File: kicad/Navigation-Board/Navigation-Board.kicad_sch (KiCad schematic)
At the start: 178 parts, among them J1 2.8" TFT, J2 0.96" OLED, J3 GME0831B, J4 Conn_01x03, SW1 SW_SPST, SW10 SW_SPST, SW11 SW_SPST, SW12 SW_SPST, SW13 SW_SPST, SW14 SW_SPST, SW15 SW_SPST, SW16 SW_SPST, SW17 SW_SPST, SW18 SW_SPST, SW19 SW_SPST, SW2 SW_SPST, SW20 SW_SPST, SW21 SW_SPST, SW22 SW_SPST, SW23 SW_SPST, SW24 SW_SPST, SW25 SW_SPST, SW26 SW_SPST, SW27 SW_SPST, SW28 SW_SPST, SW29 SW_SPST, SW3 SW_SPST, SW30 SW_SPST, SW31 SW_SPST, SW32 SW_SPST, SW33 SW_SPST, SW34 SW_SPST, SW35 SW_SPST, SW36 SW_SPST, SW37 SW_SPST, SW38 SW_SPST, SW39 SW_SPST, SW4 SW_SPST, SW40 SW_SPST, SW41 SW_SPST, SW42 SW_SPST, SW43 SW_SPST, SW44 SW_SPST, SW45 SW_SPST, SW46 SW_SPST, SW47 SW_SPST, SW48 SW_SPST, SW49 SW_SPST, SW5 SW_SPST, SW50 SW_SPST, SW51 SW_SPST, SW52 SW_SPST, SW53 SW_SPST, SW54 SW_SPST, SW55 SW_SPST, SW56 SW_SPST, SW57 SW_SPST, SW58 SW_SPST, SW59 SW_SPST, SW6 SW_SPST, SW60 SW_SPST, SW61 SW_SPST, SW62 SW_SPST, SW63 SW_SPST, SW64 SW_SPST, SW65 SW_SPST, SW66 SW_SPST, SW67 SW_SPST, SW68 SW_SPST, SW69 SW_SPST, SW7 SW_SPST, SW70 SW_SPST, SW71 SW_SPST, SW72 SW_SPST, SW73 SW_SPST, SW74 SW_SPST, SW75 SW_SPST, SW76 SW_SPST, SW77 SW_SPST, SW78 SW_SPST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

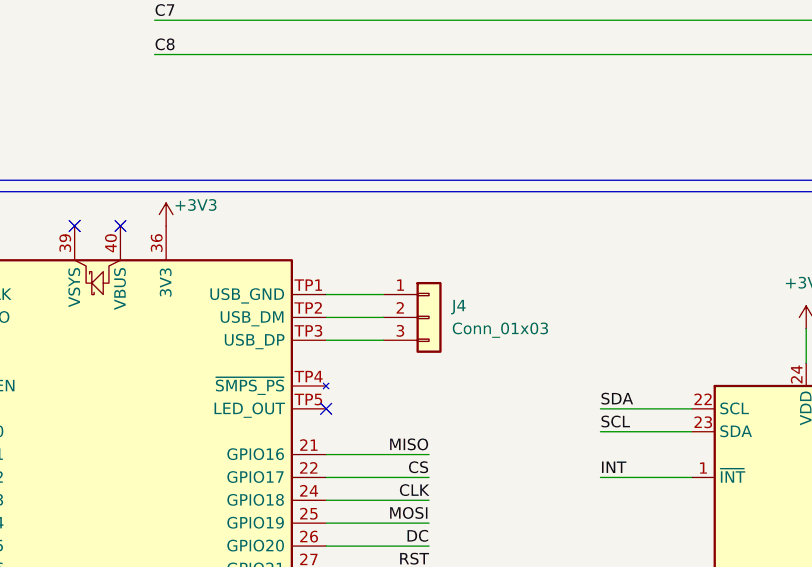
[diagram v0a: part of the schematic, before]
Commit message: made overall schematic
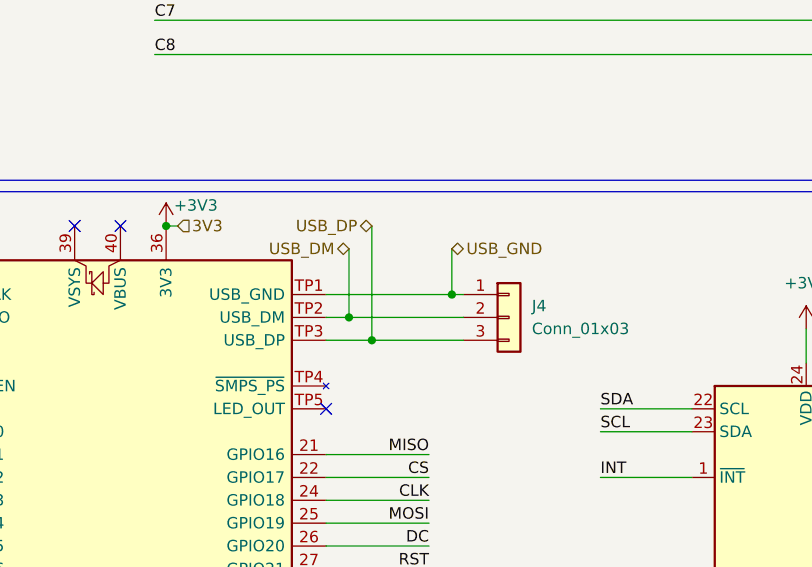
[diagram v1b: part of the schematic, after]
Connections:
- net USB_GND: now reaches A1.TP1 (USB_GND), J4.1 (Pin_1)
- net USB_DM: now reaches A1.TP2 (USB_DM), J4.2 (Pin_2)
- net USB_DP: now reaches A1.TP3 (USB_DP), J4.3 (Pin_3)
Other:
- moved on the sheet: J4
